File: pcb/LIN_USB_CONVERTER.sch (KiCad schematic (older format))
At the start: 32 parts, among them J1 Conn_01x03, J2 Conn_01x03, J3 GS2, J4 USB_A, J5 Conn_01x02, P2 CONN_01X05, U1 TJA1028, U2 MAX12931, U3 MCP1700T-3302E/TT, U4 STM32F042G4U6

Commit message: Kicad update
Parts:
- C1, C2: symbol CP1_Small -> LIN_USB_CONVERTER-rescue:CP1_Small-RESCUE-LIN_USB_CONVERTER
- C3, C4, C5, C6, C8, C9: symbol C -> LIN_USB_CONVERTER-rescue:C-RESCUE-LIN_USB_CONVERTER
- D1, D3: symbol D_Small_ALT -> LIN_USB_CONVERTER-rescue:D_Small_ALT-RESCUE-LIN_USB_CONVERTER
- D2: symbol D_Schottky_Small_ALT -> LIN_USB_CONVERTER-rescue:D_Schottky_Small_ALT-RESCUE-LIN_USB_CONVERTER
- J1, J2: symbol Conn_01x03 -> LIN_USB_CONVERTER-rescue:Conn_01x03-RESCUE-LIN_USB_CONVERTER
- J3: symbol GS2 -> LIN_USB_CONVERTER-rescue:GS2-RESCUE-LIN_USB_CONVERTER
- J4: symbol USB_A -> LIN_USB_CONVERTER-rescue:USB_A-RESCUE-LIN_USB_CONVERTER
- J5: symbol Conn_01x02 -> LIN_USB_CONVERTER-rescue:Conn_01x02-RESCUE-LIN_USB_CONVERTER
- P2: symbol CONN_01X05 -> LIN_USB_CONVERTER-rescue:CONN_01X05-RESCUE-LIN_USB_CONVERTER
- R1, R2, R3, R4, R5, R6, R7, R8: symbol R -> LIN_USB_CONVERTER-rescue:R-RESCUE-LIN_USB_CONVERTER
- U1: symbol TJA1028 -> LIN_USB_CONVERTER-rescue:TJA1028-RESCUE-LIN_USB_CONVERTER
- U2: symbol MAX12931 -> LIN_USB_CONVERTER-rescue:MAX12931-RESCUE-LIN_USB_CONVERTER
- U3: symbol MCP1700T-3302E/TT -> LIN_USB_CONVERTER-rescue:MCP1700T-3302E_TT-RESCUE-LIN_USB_CONVERTER
- U4: symbol STM32F042C6T6 -> LIN_USB_CONVERTER-rescue:STM32F042C6T6-RESCUE-LIN_USB_CONVERTER
- f1, f2, mh1: symbol fiducial -> LIN_USB_CONVERTER-rescue:fiducial-RESCUE-LIN_USB_CONVERTER
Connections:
- wire segments 58 -> 74

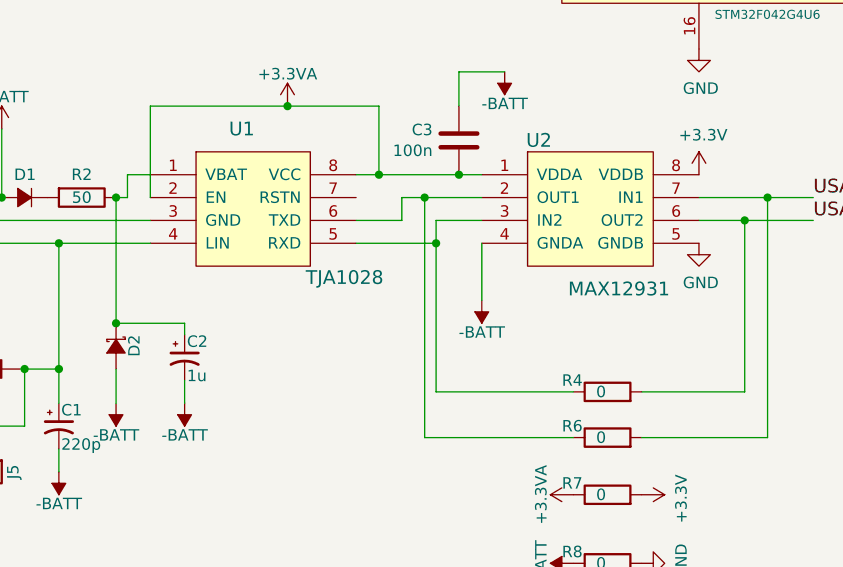
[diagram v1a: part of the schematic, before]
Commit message: Naming update
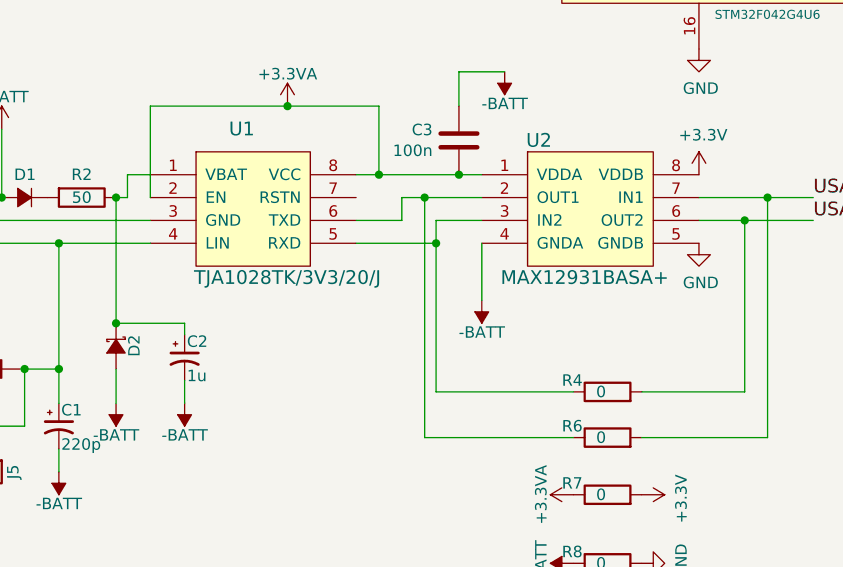
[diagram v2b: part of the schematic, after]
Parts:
- C1: 1st Disrtib Link (none) -> https://www.tme.eu/pl/details/vj0603y221kxacw2bc/kondensato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; Manufacturer (none) -> VISHAY/VJ0603Y221KXACW2BC
- C2: 1st Disrtib Link (none) -> https://www.tme.eu/pl/details/cl10b105ka8nnnc/kondensatory-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; Manufacturer (none) -> SAMSUNG/CL10B105KA8NNNC
- C3, C4, C5, C6, C9: 1st Disrtib Link (none) -> https://www.tme.eu/pl/details/c0402c104k8pac/kondensatory-m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; Manufacturer (none) -> KEMET/C0402C104K8PACTU
- C8: 1st Disrtib Link (none) -> https://www.tme.eu/pl/details/cl05b103ka5nnnc/kondensatory-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; Manufacturer (none) -> SAMSUNG/CL05B103KA5NNNC
- D1, D3: 1st Disrtib Link (none) -> https://www.tme.eu/pl/details/smbd914e6327htsa1/diody-uniwe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; Manufacturer (none) -> INFINEON
- J1: 1st Disrtib Link (none) -> https://www.tme.eu/pl/details/zl201-03g/listwy-i-gniazda-ko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; Manufacturer (none) -> CONNFLY/DS1021-1*3SF1-1
- J2: value Conn_01x03 -> TerminalBlock; 1st Disrtib Link (none) -> https://www.tme.eu/pl/details/tb-5.0-p-3p_gy/listwy-zacisko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; Manufacturer (none) -> NINIGI/TB-5.0-P-3P/GY
- J4: 1st Disrtib Link (none) -> https://www.maritex.com.pl/zlacza/zlacza_usb_hdmi_ieee/zlac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; Manufacturer (none) -> CVILUX/CU01PAH0000
- R1: 1st Disrtib Link (none) -> https://www.tme.eu/pl/details/smd0603-1k/rezystory-smd-0603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; Manufacturer (none) -> ROYAL OHM/0603SAJ0102T5E
- R2: 1st Disrtib Link (none) -> https://www.tme.eu/pl/details/rc0603fr-0749r9l/rezystory-sm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; Manufacturer (none) -> YAGEO/RC0603FR-0749R9L
- R3, R5: 1st Disrtib Link (none) -> https://www.tme.eu/pl/details/wf06p-10k-5%25/rezystory-smd-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; Manufacturer (none) -> WALSIN/WF06P103JTL
- U1: value TJA1028 -> TJA1028TK/3V3/20/J; 1st Disrtib Link (none) -> https://octopart.com/tja1028tk%2F3v3%2F20%2Fj-nxp+semicondu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; Manufacturer (none) -> NXP
- U2: value MAX12931 -> MAX12931BASA+; 1st Disrtib Link (none) -> https://octopart.com/max12931basa%2B-maxim+integrated-81881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; Manufacturer (none) -> Maxim
- U3: 1st Disrtib Link (none) -> https://octopart.com/mcp1700t-3302e%2Ftt-microchip-535742?r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; Manufacturer (none) -> Microchip
- U4: Manufacturer (none) -> ST
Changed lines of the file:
@@
 F 2 "Resistors_SMD:R_0603" H 2330 1541 50  0001 R CNN
 F 3 "" H 2400 1450 50  0000 C CNN
+F 4 "https://www.tme.eu/pl/details/wf06p-10k-5%25/rezystory-smd-0603/walsin/wf06p103jtl/" H 2400 1450 50  0001 C CNN "1st Disrtib Link"
+F 5 "WALSIN/WF06P103JTL" H 2400 1450 50  0001 C CNN "Manufacturer"
 	1    2400 1450
 	-1   0    0    1
@@
 F 2 "Capacitors_SMD:C_0402" H 5238 2800 50  0001 C CNN
 F 3 "" H 5200 2950 50  0000 C CNN
+F 4 "https://www.tme.eu/pl/details/cl05b103ka5nnnc/kondensatory-mlcc-smd-0402/samsung/" H 5200 2950 50  0001 C CNN "1st Disrtib Link"
+F 5 "SAMSUNG/CL05B103KA5NNNC" H 5200 2950 50  0001 C CNN "Manufacturer"
 	1    5200 2950
 	1    0    0    -1
@@
 F 2 "Capacitors_SMD:C_0402" H 5638 2800 50  0001 C CNN
 F 3 "" H 5600 2950 50  0000 C CNN
+F 4 "https://www.tme.eu/pl/details/c0402c104k8pac/kondensatory-mlcc-smd-0402/kemet/c0402c104k8pactu/" H 5600 2950 50  0001 C CNN "1st Disrtib Link"
+F 5 "KEMET/C0402C104K8PACTU" H 5600 2950 50  0001 C CNN "Manufacturer"
 	1    5600 2950
 	1    0    0    -1
@@
 F 2 "usb_ccb_custom:ST_UFQFPN-28_3x3mm_P0.5mm" H 5050 400 60  0001 C CNN
 F 3 "" H 3900 1600 60  0000 C CNN
-F 4 "STM32F042G4U6" H 3900 1600 60  0001 C CNN "MFG Part Num"
-F 5 "ST" H 3900 1600 60  0001 C CNN "MFG"
-F 6 "http://www.tme.eu/pl/details/stm32f042g4u6/mikrokontrolery-st/st-microelectronics/" H 3900 1600 60  0001 C CNN "1st Disrtib Link"
+F 4 "http://www.tme.eu/pl/details/stm32f042g4u6/mikrokontrolery-st/st-microelectronics/" H 3900 1600 60  0001 C CNN "1st Disrtib Link"
+F 5 "ST" H 3900 1600 50  0001 C CNN "Manufacturer"
+F 6 "STM32F042G4U6" H 3900 1600 60  0001 C CNN "MFG Part Num"
+F 7 "ST" H 3900 1600 60  0001 C CNN "MFG"
 	1    3900 1600
 	1    0    0    -1
@@
 P 2250 3550
 F 0 "U1" H 2250 3950 60  0000 C CNN
-F 1 "TJA1028" H 2700 3300 60  0000 C CNN
+F 1 "TJA1028TK/3V3/20/J" H 2450 3300 60  0000 C CNN
 F 2 "usb_ccb_custom:HVSON8" H 2250 3550 60  0001 C CNN
 F 3 "" H 2250 3550 60  0001 C CNN
+F 4 "https://octopart.com/tja1028tk%2F3v3%2F20%2Fj-nxp+semiconductors-30964986?r=sp&s=ng-i0gkdTdmf8j_7SG9MMg" H 2250 3550 50  0001 C CNN "1st Disrtib Link"
+F 5 "NXP" H 2250 3550 50  0001 C CNN "Manufacturer"
 	1    2250 3550
 	1    0    0    -1
@@
 P 700 3550
 F 0 "J2" H 700 3350 50  0000 C CNN
-F 1 "Conn_01x03" H 700 3350 50  0001 C CNN
+F 1 "TerminalBlock" H 700 3350 50  0001 C CNN
 F 2 "Connectors_Terminal_Blocks:TerminalBlock_Altech_AK300-3_P5.00mm" H 700 3550 50  0001 C CNN
 F 3 "" H 700 3550 50  0001 C CNN
+F 4 "https://www.tme.eu/pl/details/tb-5.0-p-3p_gy/listwy-zaciskowe-do-druku/ninigi/" H 700 3550 50  0001 C CNN "1st Disrtib Link"
+F 5 "NINIGI/TB-5.0-P-3P/GY" H 700 3550 50  0001 C CNN "Manufacturer"
 	1    700  3550
 	-1   0    0    1
@@
 F 2 "Resistors_SMD:R_0603" V 1480 3450 50  0001 C CNN
 F 3 "" H 1550 3450 50  0001 C CNN
+F 4 "https://www.tme.eu/pl/details/rc0603fr-0749r9l/rezystory-smd-0603/yageo/" H 1550 3450 50  0001 C CNN "1st Disrtib Link"
+F 5 "YAGEO/RC0603FR-0749R9L" H 1550 3450 50  0001 C CNN "Manufacturer"
 	1    1550 3450
 	0    1    1    0
@@
 P 3750 3500
 F 0 "U2" H 3550 3800 60  0000 C CNN
-F 1 "MAX12931" H 3900 3150 60  0000 C CNN
+F 1 "MAX12931BASA+" H 3750 3200 60  0000 C CNN
 F 2 "usb_ccb_custom:SOIC-8-N_MAXIM" H 3750 3500 60  0001 C CNN
 F 3 "" H 3750 3500 60  0001 C CNN
+F 4 "https://octopart.com/max12931basa%2B-maxim+integrated-81881677?r=sp&s=gGYYW1lERgCmIqeXABfzjw" H 3750 3500 50  0001 C CNN "1st Disrtib Link"
+F 5 "Maxim" H 3750 3500 50  0001 C CNN "Manufacturer"
 	1    3750 3500
 	1    0    0    -1
@@
 F 2 "Capacitors_SMD:C_0603" H 2000 4150 50  0001 C CNN
 F 3 "" H 2000 4150 50  0001 C CNN
+F 4 "https://www.tme.eu/pl/details/cl10b105ka8nnnc/kondensatory-mlcc-smd-0603/samsung/" H 2000 4150 50  0001 C CNN "1st Disrtib Link"
+F 5 "SAMSUNG/CL10B105KA8NNNC" H 2000 4150 50  0001 C CNN "Manufacturer"
 	1    2000 4150
 	1    0    0    -1
@@
 F 2 "Diodes_SMD:D_SOT-23_ANK" V 1300 3450 50  0001 C CNN
 F 3 "" V 1300 3450 50  0001 C CNN
+F 4 "https://www.tme.eu/pl/details/smbd914e6327htsa1/diody-uniwersalne-smd/infineon-technologies/" H 1300 3450 50  0001 C CNN "1st Disrtib Link"
+F 5 "INFINEON " H 1300 3450 50  0001 C CNN "Manufacturer"
 	1    1300 3450
 	-1   0    0    1
@@
 F 2 "Resistors_SMD:R_0603" V 5480 1250 50  0001 C CNN
 F 3 "" H 5550 1250 50  0001 C CNN
+F 4 "https://www.tme.eu/pl/details/wf06p-10k-5%25/rezystory-smd-0603/walsin/wf06p103jtl/" H 5550 1250 50  0001 C CNN "1st Disrtib Link"
+F 5 "WALSIN/WF06P103JTL" H 5550 1250 50  0001 C CNN "Manufacturer"
 	1    5550 1250
 	-1   0    0    1
@@
 F 2 "Capacitors_SMD:C_0603" H 1450 4450 50  0001 C CNN
 F 3 "" H 1450 4450 50  0001 C CNN
+F 4 "https://www.tme.eu/pl/details/vj0603y221kxacw2bc/kondensatory-mlcc-smd-0603/vishay/" H 1450 4450 50  0001 C CNN "1st Disrtib Link"
+F 5 "VISHAY/VJ0603Y221KXACW2BC" H 1450 4450 50  0001 C CNN "Manufacturer"
 	1    1450 4450
 	1    0    0    -1
@@
 F 2 "Resistors_SMD:R_0603" V 680 4200 50  0001 C CNN
 F 3 "" H 750 4200 50  0001 C CNN
+F 4 "https://www.tme.eu/pl/details/smd0603-1k/rezystory-smd-0603/royal-ohm/0603saj0102t5e/" H 750 4200 50  0001 C CNN "1st Disrtib Link"
+F 5 "ROYAL OHM/0603SAJ0102T5E" H 750 4200 50  0001 C CNN "Manufacturer"
 	1    750  4200
 	0    1    1    0
@@
 F 2 "usb_ccb_custom:USB_A_DS1097R" H 6650 2150 50  0001 C CNN
 F 3 "" H 6650 2150 50  0001 C CNN
+F 4 "https://www.maritex.com.pl/zlacza/zlacza_usb_hdmi_ieee/zlacza_i_kable_usb/wtyk_usb_1xa4_katowy/usbp1arw-cv.html" H 6500 2200 50  0001 C CNN "1st Disrtib Link"
+F 5 "CVILUX/CU01PAH0000 " H 6500 2200 50  0001 C CNN "Manufacturer"
 	1    6500 2200
 	-1   0    0    -1
@@
 F 2 "TO_SOT_Packages_SMD:SOT-23" H 10400 1104 60  0001 C CNN
 F 3 "" H 10350 1400 60  0000 C CNN
+F 4 "https://octopart.com/mcp1700t-3302e%2Ftt-microchip-535742?r=sp&s=7X4ED658TtW6VxzY9__15g" H 10350 1400 50  0001 C CNN "1st Disrtib Link"
+F 5 "Microchip" H 10350 1400 50  0001 C CNN "Manufacturer"
 	1    10350 1400
 	1    0    0    -1
@@
 F 2 "Capacitors_SMD:C_0402" H 9988 1350 50  0001 C CNN
 F 3 "" H 9950 1500 50  0000 C CNN
+F 4 "https://www.tme.eu/pl/details/c0402c104k8pac/kondensatory-mlcc-smd-0402/kemet/c0402c104k8pactu/" H 9950 1500 50  0001 C CNN "1st Disrtib Link"
+F 5 "KEMET/C0402C104K8PACTU" H 9950 1500 50  0001 C CNN "Manufacturer"
 	1    9950 1500
 	-1   0    0    -1
@@
 F 2 "Capacitors_SMD:C_0402" H 10788 1350 50  0001 C CNN
 F 3 "" H 10750 1500 50  0000 C CNN
+F 4 "https://www.tme.eu/pl/details/c0402c104k8pac/kondensatory-mlcc-smd-0402/kemet/c0402c104k8pactu/" H 10750 1500 50  0001 C CNN "1st Disrtib Link"
+F 5 "KEMET/C0402C104K8PACTU" H 10750 1500 50  0001 C CNN "Manufacturer"
 	1    10750 1500
 	1    0    0    -1
@@
 F 2 "Pin_Headers:Pin_Header_Straight_1x03_Pitch2.54mm" H 700 3150 50  0001 C CNN
 F 3 "" H 700 3150 50  0001 C CNN
+F 4 "https://www.tme.eu/pl/details/zl201-03g/listwy-i-gniazda-kolkowe/connfly/ds1021-1_3sf1-1/" H 700 3150 50  0001 C CNN "1st Disrtib Link"
+F 5 "CONNFLY/DS1021-1*3SF1-1" H 700 3150 50  0001 C CNN "Manufacturer"
 	1    700  3150
 	-1   0    0    1
@@
 F 2 "Capacitors_SMD:C_0402" H 3238 3050 50  0001 C CNN
 F 3 "" H 3200 3200 50  0000 C CNN
+F 4 "https://www.tme.eu/pl/details/c0402c104k8pac/kondensatory-mlcc-smd-0402/kemet/c0402c104k8pactu/" H 3200 3200 50  0001 C CNN "1st Disrtib Link"
+F 5 "KEMET/C0402C104K8PACTU" H 3200 3200 50  0001 C CNN "Manufacturer"
 	1    3200 3200
 	-1   0    0    -1
@@
 F 2 "Capacitors_SMD:C_0402" H 6138 2800 50  0001 C CNN
 F 3 "" H 6100 2950 50  0000 C CNN
+F 4 "https://www.tme.eu/pl/details/c0402c104k8pac/kondensatory-mlcc-smd-0402/kemet/c0402c104k8pactu/" H 6100 2950 50  0001 C CNN "1st Disrtib Link"
+F 5 "KEMET/C0402C104K8PACTU" H 6100 2950 50  0001 C CNN "Manufacturer"
 	1    6100 2950
 	1    0    0    -1
@@
 F 2 "Diodes_SMD:D_SOT-23_ANK" V 600 4050 50  0001 C CNN
 F 3 "" V 600 4050 50  0001 C CNN
+F 4 "https://www.tme.eu/pl/details/smbd914e6327htsa1/diody-uniwersalne-smd/infineon-technologies/" H 600 4050 50  0001 C CNN "1st Disrtib Link"
+F 5 "INFINEON " H 600 4050 50  0001 C CNN "Manufacturer"
 	1    600  4050
 	0    1    1    0

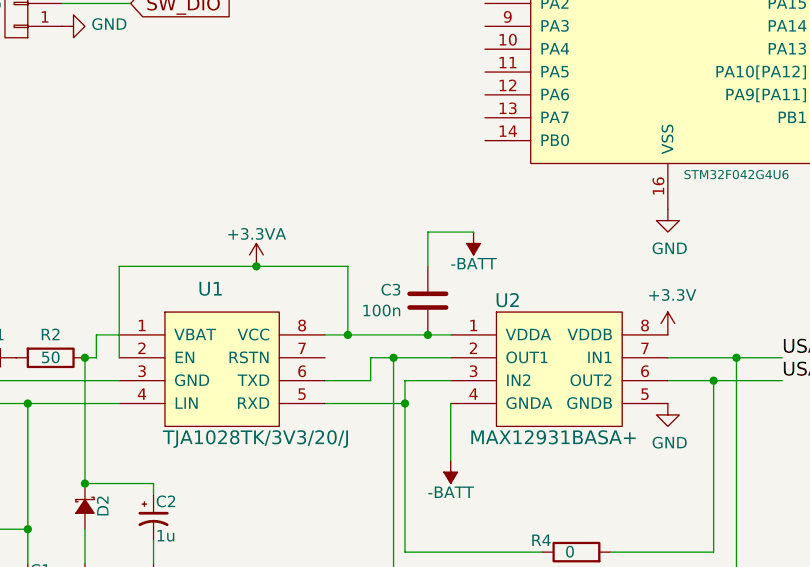
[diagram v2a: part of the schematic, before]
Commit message: PCB release
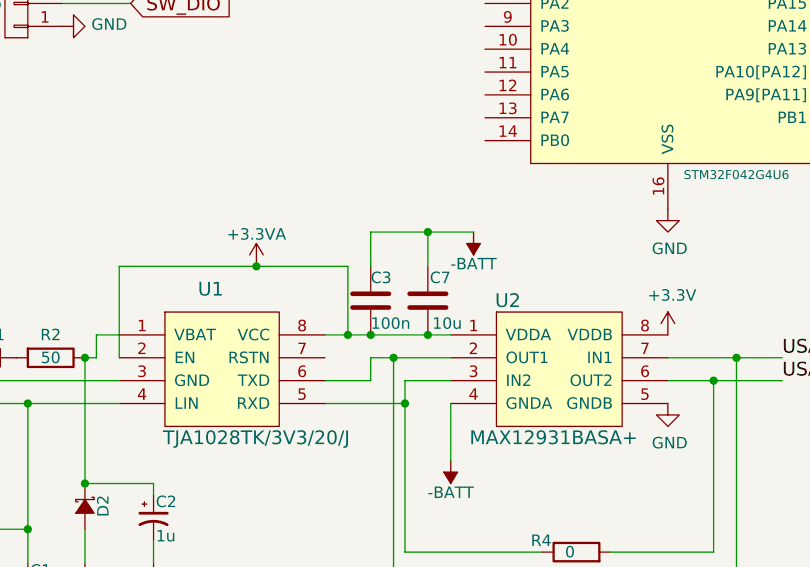
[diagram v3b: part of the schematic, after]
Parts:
- added C3: 100n, Capacitors_SMD:C_0402, symbol LIN_USB_CONVERTER-rescue:C-RESCUE-LIN_USB_CONVERTER
- C7: renamed from C3; value 100n -> 10u; 1st Disrtib Link https://www.tme.eu/pl/details/c0402c104k8pac/kondensatory-m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 -> https://www.tme.eu/pl/details/cl05a106mq5nunc/kondensatory-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; Manufacturer KEMET/C0402C104K8PACTU -> SAMSUNG/CL05A106MQ5NUNC
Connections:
- net +3.3VA: now also C3.2
- net -BATT: now also C3.1
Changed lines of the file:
@@
 $EndComp
 $Comp
-L LIN_USB_CONVERTER-rescue:C-RESCUE-LIN_USB_CONVERTER C3
+L LIN_USB_CONVERTER-rescue:C-RESCUE-LIN_USB_CONVERTER C7
 U 1 1 5A6A648D
 P 3200 3200
-F 0 "C3" H 3315 3246 50  0000 L CNN
-F 1 "100n" H 3315 3155 50  0000 L CNN
+F 0 "C7" H 3100 3300 50  0000 L CNN
+F 1 "10u" H 3050 3100 50  0000 L CNN
 F 2 "Capacitors_SMD:C_0402" H 3238 3050 50  0001 C CNN
 F 3 "" H 3200 3200 50  0000 C CNN
-F 4 "https://www.tme.eu/pl/details/c0402c104k8pac/kondensatory-mlcc-smd-0402/kemet/c0402c104k8pactu/" H 3200 3200 50  0001 C CNN "1st Disrtib Link"
-F 5 "KEMET/C0402C104K8PACTU" H 3200 3200 50  0001 C CNN "Manufacturer"
+F 4 "https://www.tme.eu/pl/details/cl05a106mq5nunc/kondensatory-mlcc-smd-0402/samsung/" H 3200 3200 50  0001 C CNN "1st Disrtib Link"
+F 5 "SAMSUNG/CL05A106MQ5NUNC" H 3200 3200 50  0001 C CNN "Manufacturer"
 	1    3200 3200
 	-1   0    0    -1
@@
 	950  3550 950  3800
 Wire Wire Line
-	3200 3350 2850 3350
-Wire Wire Line
 	2450 3050 2850 3050
 Wire Wire Line
@@
 Wire Wire Line
 	4450 3550 4750 3550
+Wire Wire Line
+	3200 2900 2950 2900
+Wire Wire Line
+	2950 2900 2950 3050
+Connection ~ 3200 2900
+Wire Wire Line
+	2850 3350 2950 3350
+$Comp
+L LIN_USB_CONVERTER-rescue:C-RESCUE-LIN_USB_CONVERTER C3
+U 1 1 5AB17A84
+P 2950 3200
+F 0 "C3" H 2950 3300 50  0000 L CNN
+F 1 "100n" H 2950 3100 50  0000 L CNN
+F 2 "Capacitors_SMD:C_0402" H 2988 3050 50  0001 C CNN
+F 3 "" H 2950 3200 50  0000 C CNN
+F 4 "https://www.tme.eu/pl/details/c0402c104k8pac/kondensatory-mlcc-smd-0402/kemet/c0402c104k8pactu/" H 2950 3200 50  0001 C CNN "1st Disrtib Link"
+F 5 "KEMET/C0402C104K8PACTU" H 2950 3200 50  0001 C CNN "Manufacturer"
+	1    2950 3200
+	1    0    0    -1
+$EndComp
+Connection ~ 2950 3350
+Wire Wire Line
+	2950 3350 3200 3350
 $EndSCHEMATC
